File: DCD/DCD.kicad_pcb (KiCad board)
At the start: 4 copper layers, 110 x 110 mm, 172 parts, among them IC1 830S21AMI-01LF, IC2 830S21AMI-01LF, J1 UMPS-04-03.5-G-VT-SM-WT, J2 UMPS-04-03.5-G-VT-SM-WT, J3 UMPS-04-03.5-G-VT-SM-WT, J4 UMPS-04-03.5-G-VT-SM-WT, J5 Conn_02x04_Top_Bottom, U1 TLV76780DBVR, U10 OPA277UA, U11 DAC8811ICDGKT, U12 DAC8811ICDGKT, U13 OPA277UA, U14 OPA277UA, U15 MC100EP31DTG, U16 MC100EP31DTG, U2 ADP7182AUJZ-1.8-R7, U3 LP2985-50DBVR, U4 LP2985-18DBVR, U5 LP2985-33DBVR, U6 ADR4550BRZ, U7 LP2985-33DBVR, U8 CDCLVC1104PWR, U9 AD4630-24BBCZ, Y1 SiT8208AI-21-33E-50.000000

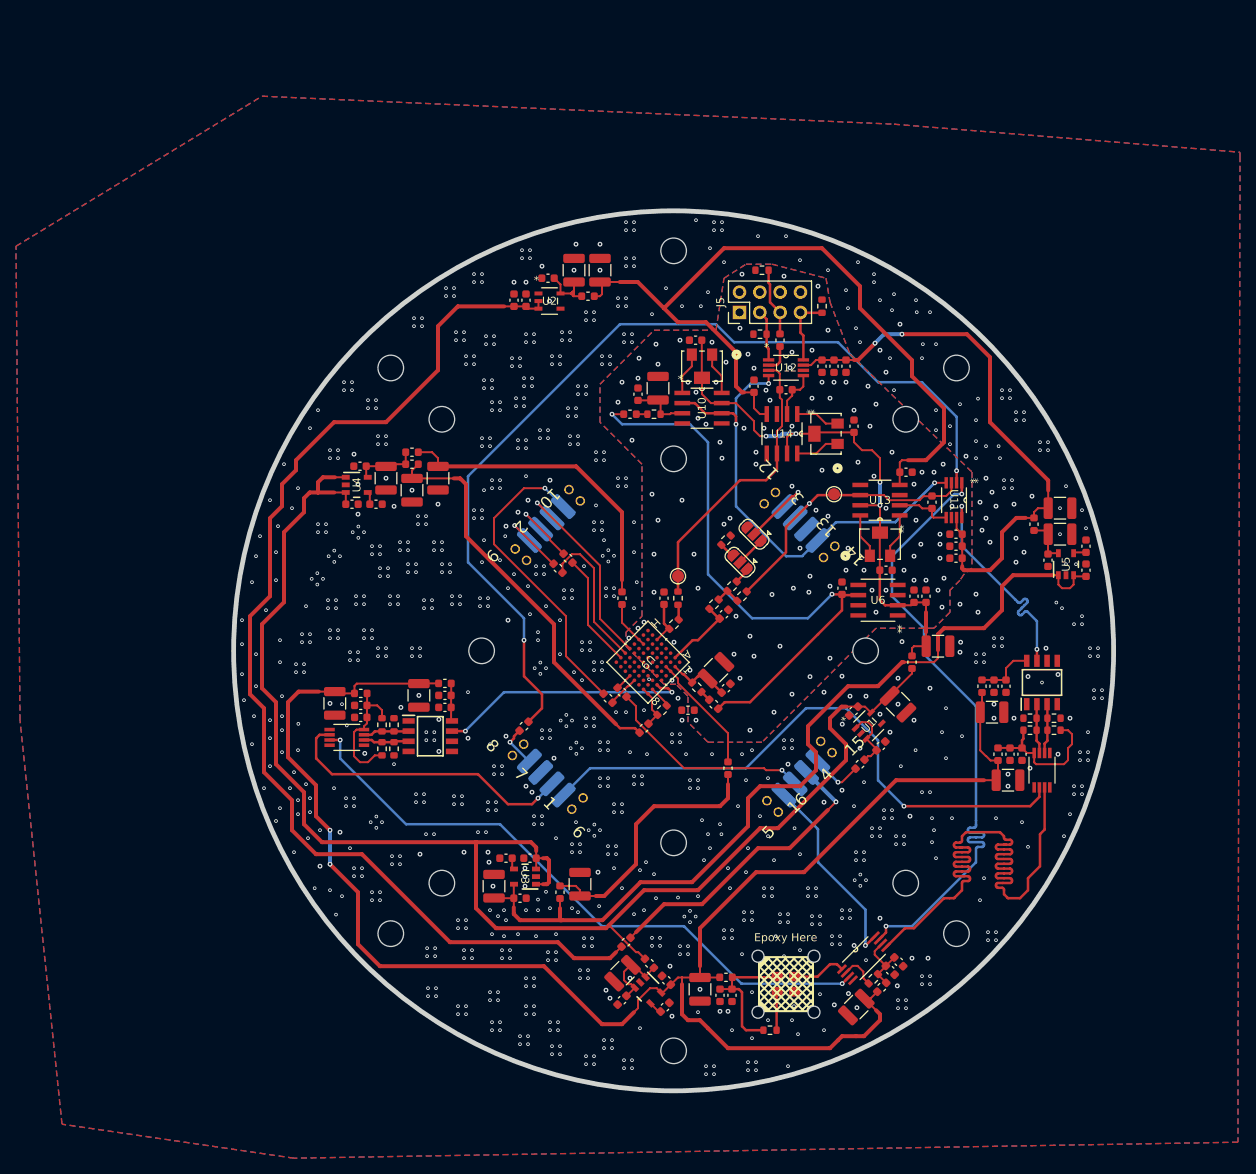
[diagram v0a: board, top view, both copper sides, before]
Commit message: Component placement
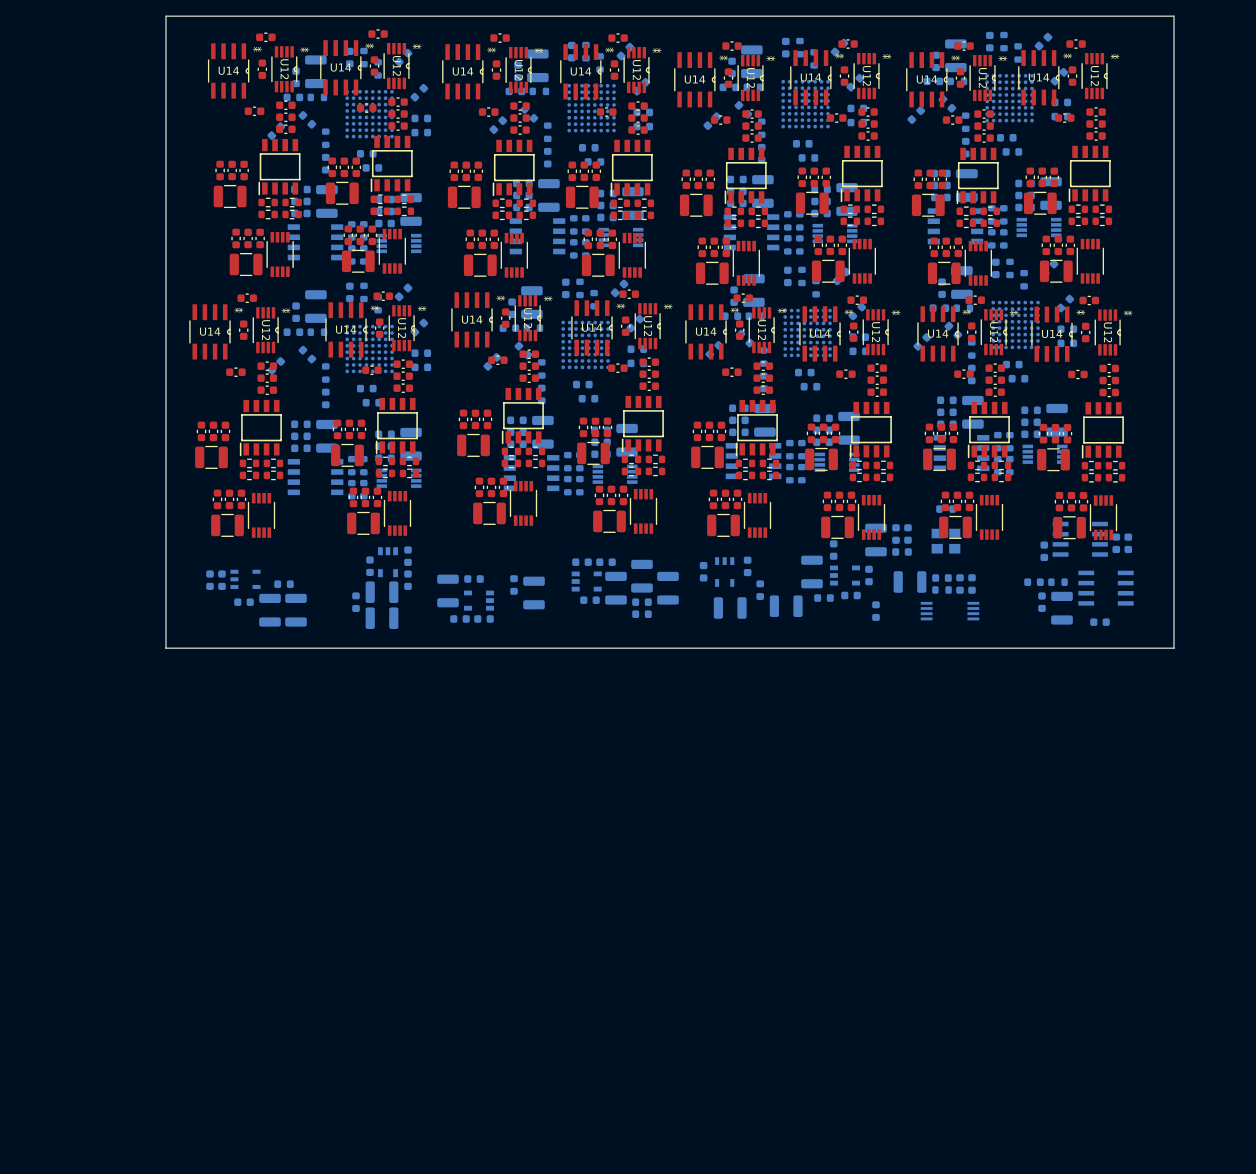
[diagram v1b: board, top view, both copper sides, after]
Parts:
- removed B1: DIN933 M3x14mm, custom_components:Screw_DIN933_M3x14mm
- removed C38: 1µF, Capacitor_SMD:C_0603_1608Metric
- removed C40: 100p, Capacitor_SMD:C_0603_1608Metric
- removed C43: 1nF, Capacitor_SMD:C_0603_1608Metric
- removed C44: 10pF, Capacitor_SMD:C_0603_1608Metric
- removed C47, C48: 100nF, Capacitor_SMD:C_0603_1608Metric
- removed FB11, FB12, FB14: 470Ω, Inductor_SMD:L_0603_1608Metric
- removed H1, H10, H11, H12, H13, H14, H2, H3, H4, H5, H6, H7, H8, H9: M3 Mounting hole, LOBSTER:MountingHole_3.2mm_M3_NoMask
- removed H15: Spacer M3x5mm, custom_components:ThreadedSpacer_6mm_M3x0.5_5mm
- removed J1, J2, J3, J4: UMPS-04-03.5-G-VT-SM-WT, custom_components:UMPS-04-03.5-G-VT-SM-WT
- removed J5: Conn_02x04_Top_Bottom, Connector_PinHeader_2.54mm:PinHeader_2x04_P2.54mm_Vertical
- removed JP1, JP2: SolderJumper_3_Open, Jumper:SolderJumper-3_P1.3mm_Open_RoundedPad1.0x1.5mm
- removed N1, N2, N3, N4, N5, N6, N7: M3 Thumbnut, custom_components:ThumbNut-M3
- removed R17: 47, Resistor_SMD:R_0603_1608Metric
- removed R18, R19, R20: 1k, Resistor_SMD:R_0603_1608Metric
- removed R3, R4, R5: 10k, Resistor_SMD:R_0603_1608Metric
- removed RV1, RV2, RV3: 20kR, custom_components:IC3_3214W-1-203E_BRN
- removed TP1, TP2: TestPoint, TestPoint:TestPoint_Pad_D1.5mm
- removed U11: DAC8811ICDGKT, custom_components:DGK8
- removed U13: OPA277UA, custom_components:D8
- added C23: 10uF, Capacitor_SMD:C_1210_3225Metric, F.Cu at (194.5, 47.6)
- added C23: 10uF, Capacitor_SMD:C_1210_3225Metric, F.Cu at (138.7, 78.9)
- added C23: 10uF, Capacitor_SMD:C_1210_3225Metric, F.Cu at (122.5, 46.9)
- added C23: 10uF, Capacitor_SMD:C_1210_3225Metric, F.Cu at (152.9, 79.4)
- added C23: 10uF, Capacitor_SMD:C_1210_3225Metric, F.Cu at (123.7, 77.9)
- added C23: 10uF, Capacitor_SMD:C_1210_3225Metric, F.Cu at (107.9, 79.2)
- added C23: 10uF, Capacitor_SMD:C_1210_3225Metric, F.Cu at (90.9, 79.4)
- added C23: 10uF, Capacitor_SMD:C_1210_3225Metric, F.Cu at (180.5, 47.9)
- added C23: 10uF, Capacitor_SMD:C_1210_3225Metric, F.Cu at (137.3, 46.9)
- added C23: 10uF, Capacitor_SMD:C_1210_3225Metric, F.Cu at (167.2, 79.7)
- added C23: 10uF, Capacitor_SMD:C_1210_3225Metric, F.Cu at (181.9, 79.7)
- added C23: 10uF, Capacitor_SMD:C_1210_3225Metric, F.Cu at (196.2, 79.7)
- added C23: 10uF, Capacitor_SMD:C_1210_3225Metric, F.Cu at (107.3, 46.4)
- added C23: 10uF, Capacitor_SMD:C_1210_3225Metric, F.Cu at (166.0, 47.6)
- added C23: 10uF, Capacitor_SMD:C_1210_3225Metric, F.Cu at (151.5, 47.9)
- added C30: 10uF, Capacitor_SMD:C_1210_3225Metric, B.Cu at (129.0, 51.5)
- added C30: 10uF, Capacitor_SMD:C_1210_3225Metric, B.Cu at (129.7, 21.9)
- added C30: 10uF, Capacitor_SMD:C_1210_3225Metric, B.Cu at (102.0, 22.7)
- added C30: 10uF, Capacitor_SMD:C_1210_3225Metric, B.Cu at (156.5, 21.4)
- added C30: 10uF, Capacitor_SMD:C_1210_3225Metric, B.Cu at (102.0, 52.0)
- added C30: 10uF, Capacitor_SMD:C_1210_3225Metric, B.Cu at (156.7, 50.0)
- added C30: 10uF, Capacitor_SMD:C_1210_3225Metric, B.Cu at (182.7, 49.0)
- added C32: 100nF, Capacitor_SMD:C_0603_1608Metric, B.Cu at (180.3, 49.8)
- added C32: 100nF, Capacitor_SMD:C_0603_1608Metric, B.Cu at (154.3, 50.8)
- added C32: 100nF, Capacitor_SMD:C_0603_1608Metric, B.Cu at (99.5, 52.8)
- added C32: 100nF, Capacitor_SMD:C_0603_1608Metric, B.Cu at (154.0, 22.2)
- added C32: 100nF, Capacitor_SMD:C_0603_1608Metric, B.Cu at (126.5, 52.2)
- added C32: 100nF, Capacitor_SMD:C_0603_1608Metric, B.Cu at (99.5, 23.4)
- added C32: 100nF, Capacitor_SMD:C_0603_1608Metric, B.Cu at (127.3, 22.7)
- added C36: 1nF, Capacitor_SMD:C_0603_1608Metric, B.Cu at (160.7, 19.7)
- added C36: 1nF, Capacitor_SMD:C_0603_1608Metric, B.Cu at (161.0, 48.3)
- added C36: 1nF, Capacitor_SMD:C_0603_1608Metric, B.Cu at (187.0, 47.3)
- added C36: 1nF, Capacitor_SMD:C_0603_1608Metric, B.Cu at (106.2, 50.3)
- added C36: 1nF, Capacitor_SMD:C_0603_1608Metric, B.Cu at (133.2, 49.8)
- added C36: 1nF, Capacitor_SMD:C_0603_1608Metric, B.Cu at (106.2, 20.9)
- added C36: 1nF, Capacitor_SMD:C_0603_1608Metric, B.Cu at (134.0, 20.2)
- added C37: 1nF, Capacitor_SMD:C_0603_1608Metric, B.Cu at (140.7, 20.2)
- added C37: 1nF, Capacitor_SMD:C_0603_1608Metric, B.Cu at (167.4, 19.7)
- added C37: 1nF, Capacitor_SMD:C_0603_1608Metric, B.Cu at (112.9, 50.3)
- added C37: 1nF, Capacitor_SMD:C_0603_1608Metric, B.Cu at (167.7, 48.3)
- added C37: 1nF, Capacitor_SMD:C_0603_1608Metric, B.Cu at (139.9, 49.8)
- added C37: 1nF, Capacitor_SMD:C_0603_1608Metric, B.Cu at (112.9, 20.9)
- added C37: 1nF, Capacitor_SMD:C_0603_1608Metric, B.Cu at (193.7, 47.3)
- added C39: 1µF, Capacitor_SMD:C_0603_1608Metric, F.Cu at (201.2, 62.8)
- added C39: 1µF, Capacitor_SMD:C_0603_1608Metric, F.Cu at (112.9, 62.2)
- added C39: 1µF, Capacitor_SMD:C_0603_1608Metric, F.Cu at (156.5, 31.0)
- added C39: 1µF, Capacitor_SMD:C_0603_1608Metric, F.Cu at (95.9, 62.5)
- added C39: 1µF, Capacitor_SMD:C_0603_1608Metric, F.Cu at (143.7, 62.0)
- added C39: 1µF, Capacitor_SMD:C_0603_1608Metric, F.Cu at (127.5, 30.0)
- added C39: 1µF, Capacitor_SMD:C_0603_1608Metric, F.Cu at (157.9, 62.5)
- added C39: 1µF, Capacitor_SMD:C_0603_1608Metric, F.Cu at (172.2, 62.7)
- added C39: 1µF, Capacitor_SMD:C_0603_1608Metric, F.Cu at (128.7, 61.0)
- added C39: 1µF, Capacitor_SMD:C_0603_1608Metric, F.Cu at (171.0, 30.7)
- added C39: 1µF, Capacitor_SMD:C_0603_1608Metric, F.Cu at (112.3, 29.5)
- added C39: 1µF, Capacitor_SMD:C_0603_1608Metric, F.Cu at (199.5, 30.7)
- added C39: 1µF, Capacitor_SMD:C_0603_1608Metric, F.Cu at (142.3, 30.0)
- added C39: 1µF, Capacitor_SMD:C_0603_1608Metric, F.Cu at (186.9, 62.7)
- added C39: 1µF, Capacitor_SMD:C_0603_1608Metric, F.Cu at (185.5, 31.0)
- added C41: 100p, Capacitor_SMD:C_0603_1608Metric, F.Cu at (112.3, 26.5)
- added C41: 100p, Capacitor_SMD:C_0603_1608Metric, F.Cu at (143.7, 59.0)
- added C41: 100p, Capacitor_SMD:C_0603_1608Metric, F.Cu at (142.3, 27.0)
- added C41: 100p, Capacitor_SMD:C_0603_1608Metric, F.Cu at (156.5, 28.0)
- added C41: 100p, Capacitor_SMD:C_0603_1608Metric, F.Cu at (157.9, 59.5)
- added C41: 100p, Capacitor_SMD:C_0603_1608Metric, F.Cu at (128.7, 58.0)
- added C41: 100p, Capacitor_SMD:C_0603_1608Metric, F.Cu at (186.9, 59.7)
- added C41: 100p, Capacitor_SMD:C_0603_1608Metric, F.Cu at (171.0, 27.7)
- added C41: 100p, Capacitor_SMD:C_0603_1608Metric, F.Cu at (112.9, 59.2)
- added C41: 100p, Capacitor_SMD:C_0603_1608Metric, F.Cu at (95.9, 59.5)
- added C41: 100p, Capacitor_SMD:C_0603_1608Metric, F.Cu at (201.2, 59.8)
- added C41: 100p, Capacitor_SMD:C_0603_1608Metric, F.Cu at (172.2, 59.7)
- added C41: 100p, Capacitor_SMD:C_0603_1608Metric, F.Cu at (127.5, 27.0)
- added C41: 100p, Capacitor_SMD:C_0603_1608Metric, F.Cu at (199.5, 27.7)
- added C41: 100p, Capacitor_SMD:C_0603_1608Metric, F.Cu at (185.5, 28.0)
- added C42: 1nF, Capacitor_SMD:C_0603_1608Metric, F.Cu at (199.5, 29.2)
- added C42: 1nF, Capacitor_SMD:C_0603_1608Metric, F.Cu at (128.7, 59.5)
- added C42: 1nF, Capacitor_SMD:C_0603_1608Metric, F.Cu at (185.5, 29.5)
- added C42: 1nF, Capacitor_SMD:C_0603_1608Metric, F.Cu at (95.9, 61.0)
- added C42: 1nF, Capacitor_SMD:C_0603_1608Metric, F.Cu at (201.2, 61.3)
- added C42: 1nF, Capacitor_SMD:C_0603_1608Metric, F.Cu at (143.7, 60.5)
- added C42: 1nF, Capacitor_SMD:C_0603_1608Metric, F.Cu at (112.9, 60.7)
- added C42: 1nF, Capacitor_SMD:C_0603_1608Metric, F.Cu at (172.2, 61.2)
- added C42: 1nF, Capacitor_SMD:C_0603_1608Metric, F.Cu at (171.0, 29.2)
- added C42: 1nF, Capacitor_SMD:C_0603_1608Metric, F.Cu at (157.9, 61.0)
- added C42: 1nF, Capacitor_SMD:C_0603_1608Metric, F.Cu at (156.5, 29.5)
- added C42: 1nF, Capacitor_SMD:C_0603_1608Metric, F.Cu at (142.3, 28.5)
- added C42: 1nF, Capacitor_SMD:C_0603_1608Metric, F.Cu at (127.5, 28.5)
- added C42: 1nF, Capacitor_SMD:C_0603_1608Metric, F.Cu at (112.3, 28.0)
- added C42: 1nF, Capacitor_SMD:C_0603_1608Metric, F.Cu at (186.9, 61.2)
- added C45: 10pF, Capacitor_SMD:C_0603_1608Metric, F.Cu at (196.6, 23.2)
- added C45: 10pF, Capacitor_SMD:C_0603_1608Metric, F.Cu at (109.3, 22.0)
- added C45: 10pF, Capacitor_SMD:C_0603_1608Metric, F.Cu at (124.6, 22.5)
- added C45: 10pF, Capacitor_SMD:C_0603_1608Metric, F.Cu at (125.7, 53.5)
- added C45: 10pF, Capacitor_SMD:C_0603_1608Metric, F.Cu at (93.0, 55.0)
- added C45: 10pF, Capacitor_SMD:C_0603_1608Metric, F.Cu at (155.0, 55.0)
- added C45: 10pF, Capacitor_SMD:C_0603_1608Metric, F.Cu at (139.3, 22.5)
- added C45: 10pF, Capacitor_SMD:C_0603_1608Metric, F.Cu at (184.0, 55.2)
- added C45: 10pF, Capacitor_SMD:C_0603_1608Metric, F.Cu at (169.2, 55.2)
- added C45: 10pF, Capacitor_SMD:C_0603_1608Metric, F.Cu at (140.7, 54.5)
- added C45: 10pF, Capacitor_SMD:C_0603_1608Metric, F.Cu at (182.6, 23.5)
- added C45: 10pF, Capacitor_SMD:C_0603_1608Metric, F.Cu at (110.0, 54.7)
- added C45: 10pF, Capacitor_SMD:C_0603_1608Metric, F.Cu at (153.6, 23.5)
- added C45: 10pF, Capacitor_SMD:C_0603_1608Metric, F.Cu at (198.2, 55.3)
- added C45: 10pF, Capacitor_SMD:C_0603_1608Metric, F.Cu at (168.1, 23.2)
- added C49: 100nF, Capacitor_SMD:C_0603_1608Metric, F.Cu at (141.2, 50.5)
- added C49: 100nF, Capacitor_SMD:C_0603_1608Metric, F.Cu at (109.8, 18.0)
- added C49: 100nF, Capacitor_SMD:C_0603_1608Metric, F.Cu at (169.7, 51.2)
- added C49: 100nF, Capacitor_SMD:C_0603_1608Metric, F.Cu at (168.5, 19.2)
- added C49: 100nF, Capacitor_SMD:C_0603_1608Metric, F.Cu at (198.7, 51.3)
- added C49: 100nF, Capacitor_SMD:C_0603_1608Metric, F.Cu at (197.0, 19.2)
- added C49: 100nF, Capacitor_SMD:C_0603_1608Metric, F.Cu at (125.0, 18.5)
- added C49: 100nF, Capacitor_SMD:C_0603_1608Metric, F.Cu at (154.0, 19.5)
- added C49: 100nF, Capacitor_SMD:C_0603_1608Metric, F.Cu at (184.4, 51.2)
- added C49: 100nF, Capacitor_SMD:C_0603_1608Metric, F.Cu at (155.4, 51.0)
- added C49: 100nF, Capacitor_SMD:C_0603_1608Metric, F.Cu at (139.8, 18.5)
- added C49: 100nF, Capacitor_SMD:C_0603_1608Metric, F.Cu at (93.4, 51.0)
- added C49: 100nF, Capacitor_SMD:C_0603_1608Metric, F.Cu at (183.0, 19.5)
- added C49: 100nF, Capacitor_SMD:C_0603_1608Metric, F.Cu at (110.4, 50.7)
- added C50: 100nF, Capacitor_SMD:C_0603_1608Metric, F.Cu at (181.6, 28.7)
- added C50: 100nF, Capacitor_SMD:C_0603_1608Metric, F.Cu at (109.0, 60.0)
- added C50: 100nF, Capacitor_SMD:C_0603_1608Metric, F.Cu at (168.2, 60.5)
- added C50: 100nF, Capacitor_SMD:C_0603_1608Metric, F.Cu at (197.2, 60.5)
- added C50: 100nF, Capacitor_SMD:C_0603_1608Metric, F.Cu at (139.7, 59.7)
- added C50: 100nF, Capacitor_SMD:C_0603_1608Metric, F.Cu at (183.0, 60.5)
- added C50: 100nF, Capacitor_SMD:C_0603_1608Metric, F.Cu at (92.0, 60.2)
- added C50: 100nF, Capacitor_SMD:C_0603_1608Metric, F.Cu at (154.0, 60.2)
- added C50: 100nF, Capacitor_SMD:C_0603_1608Metric, F.Cu at (108.3, 27.2)
- added C50: 100nF, Capacitor_SMD:C_0603_1608Metric, F.Cu at (138.3, 27.7)
- added C50: 100nF, Capacitor_SMD:C_0603_1608Metric, F.Cu at (123.6, 27.7)
- added C50: 100nF, Capacitor_SMD:C_0603_1608Metric, F.Cu at (167.1, 28.5)
- added C50: 100nF, Capacitor_SMD:C_0603_1608Metric, F.Cu at (195.6, 28.5)
- added C50: 100nF, Capacitor_SMD:C_0603_1608Metric, F.Cu at (124.7, 58.7)
- added C50: 100nF, Capacitor_SMD:C_0603_1608Metric, F.Cu at (152.6, 28.7)
- added C59: 1µF, Capacitor_SMD:C_0603_1608Metric, F.Cu at (138.9, 75.7)
- added C59: 1µF, Capacitor_SMD:C_0603_1608Metric, F.Cu at (182.2, 76.4)
- added C59: 1µF, Capacitor_SMD:C_0603_1608Metric, F.Cu at (167.4, 76.4)
- added C59: 1µF, Capacitor_SMD:C_0603_1608Metric, F.Cu at (151.8, 44.6)
- added C59: 1µF, Capacitor_SMD:C_0603_1608Metric, F.Cu at (180.8, 44.6)
- added C59: 1µF, Capacitor_SMD:C_0603_1608Metric, F.Cu at (108.2, 75.9)
- added C59: 1µF, Capacitor_SMD:C_0603_1608Metric, F.Cu at (137.5, 43.6)
- added C59: 1µF, Capacitor_SMD:C_0603_1608Metric, F.Cu at (153.2, 76.2)
- added C59: 1µF, Capacitor_SMD:C_0603_1608Metric, F.Cu at (123.9, 74.7)
- added C59: 1µF, Capacitor_SMD:C_0603_1608Metric, F.Cu at (91.2, 76.2)
- added C59: 1µF, Capacitor_SMD:C_0603_1608Metric, F.Cu at (194.8, 44.4)
- added C59: 1µF, Capacitor_SMD:C_0603_1608Metric, F.Cu at (107.5, 43.1)
- added C59: 1µF, Capacitor_SMD:C_0603_1608Metric, F.Cu at (122.8, 43.6)
- added C59: 1µF, Capacitor_SMD:C_0603_1608Metric, F.Cu at (196.4, 76.4)
- added C59: 1µF, Capacitor_SMD:C_0603_1608Metric, F.Cu at (166.3, 44.4)
- added C60: 100nF, Capacitor_SMD:C_0603_1608Metric, F.Cu at (153.3, 44.6)
- added C60: 100nF, Capacitor_SMD:C_0603_1608Metric, F.Cu at (92.7, 76.2)
- added C60: 100nF, Capacitor_SMD:C_0603_1608Metric, F.Cu at (167.8, 44.4)
- added C60: 100nF, Capacitor_SMD:C_0603_1608Metric, F.Cu at (109.0, 43.1)
- added C60: 100nF, Capacitor_SMD:C_0603_1608Metric, F.Cu at (139.0, 43.6)
- added C60: 100nF, Capacitor_SMD:C_0603_1608Metric, F.Cu at (109.7, 75.9)
- added C60: 100nF, Capacitor_SMD:C_0603_1608Metric, F.Cu at (140.4, 75.7)
- added C60: 100nF, Capacitor_SMD:C_0603_1608Metric, F.Cu at (124.3, 43.6)
- added C60: 100nF, Capacitor_SMD:C_0603_1608Metric, F.Cu at (183.7, 76.4)
- added C60: 100nF, Capacitor_SMD:C_0603_1608Metric, F.Cu at (154.7, 76.2)
- added C60: 100nF, Capacitor_SMD:C_0603_1608Metric, F.Cu at (197.9, 76.4)
- added C60: 100nF, Capacitor_SMD:C_0603_1608Metric, F.Cu at (168.9, 76.4)
- added C60: 100nF, Capacitor_SMD:C_0603_1608Metric, F.Cu at (196.3, 44.4)
- added C60: 100nF, Capacitor_SMD:C_0603_1608Metric, F.Cu at (125.4, 74.7)
- added C60: 100nF, Capacitor_SMD:C_0603_1608Metric, F.Cu at (182.3, 44.6)
- added C61: 10uF, Capacitor_SMD:C_1210_3225Metric, F.Cu at (136.7, 70.4)
- added C61: 10uF, Capacitor_SMD:C_1210_3225Metric, F.Cu at (120.5, 38.4)
- added C61: 10uF, Capacitor_SMD:C_1210_3225Metric, F.Cu at (149.5, 39.4)
- added C61: 10uF, Capacitor_SMD:C_1210_3225Metric, F.Cu at (88.9, 70.9)
- added C61: 10uF, Capacitor_SMD:C_1210_3225Metric, F.Cu at (121.7, 69.4)
- added C61: 10uF, Capacitor_SMD:C_1210_3225Metric, F.Cu at (178.5, 39.4)
- added C61: 10uF, Capacitor_SMD:C_1210_3225Metric, F.Cu at (135.3, 38.4)
- added C61: 10uF, Capacitor_SMD:C_1210_3225Metric, F.Cu at (165.2, 71.2)
- added C61: 10uF, Capacitor_SMD:C_1210_3225Metric, F.Cu at (105.3, 37.9)
- added C61: 10uF, Capacitor_SMD:C_1210_3225Metric, F.Cu at (179.9, 71.2)
- added C61: 10uF, Capacitor_SMD:C_1210_3225Metric, F.Cu at (150.9, 70.9)
- added C61: 10uF, Capacitor_SMD:C_1210_3225Metric, F.Cu at (105.9, 70.7)
- added C61: 10uF, Capacitor_SMD:C_1210_3225Metric, F.Cu at (164.0, 39.1)
- added C61: 10uF, Capacitor_SMD:C_1210_3225Metric, F.Cu at (194.2, 71.2)
- added C61: 10uF, Capacitor_SMD:C_1210_3225Metric, F.Cu at (192.5, 39.1)
- added C62: 1µF, Capacitor_SMD:C_0603_1608Metric, F.Cu at (151.2, 67.7)
- added C62: 1µF, Capacitor_SMD:C_0603_1608Metric, F.Cu at (105.5, 34.6)
- added C62: 1µF, Capacitor_SMD:C_0603_1608Metric, F.Cu at (120.8, 35.1)
- added C62: 1µF, Capacitor_SMD:C_0603_1608Metric, F.Cu at (89.2, 67.7)
- added C62: 1µF, Capacitor_SMD:C_0603_1608Metric, F.Cu at (165.4, 67.9)
- added C62: 1µF, Capacitor_SMD:C_0603_1608Metric, F.Cu at (192.8, 35.9)
- added C62: 1µF, Capacitor_SMD:C_0603_1608Metric, F.Cu at (194.4, 67.9)
- added C62: 1µF, Capacitor_SMD:C_0603_1608Metric, F.Cu at (178.8, 36.1)
- added C62: 1µF, Capacitor_SMD:C_0603_1608Metric, F.Cu at (106.2, 67.4)
- added C62: 1µF, Capacitor_SMD:C_0603_1608Metric, F.Cu at (121.9, 66.2)
- added C62: 1µF, Capacitor_SMD:C_0603_1608Metric, F.Cu at (135.5, 35.1)
- added C62: 1µF, Capacitor_SMD:C_0603_1608Metric, F.Cu at (149.8, 36.1)
- added C62: 1µF, Capacitor_SMD:C_0603_1608Metric, F.Cu at (164.3, 35.9)
- added C62: 1µF, Capacitor_SMD:C_0603_1608Metric, F.Cu at (180.2, 67.9)
- added C62: 1µF, Capacitor_SMD:C_0603_1608Metric, F.Cu at (136.9, 67.2)
- added C63: 100nF, Capacitor_SMD:C_0603_1608Metric, F.Cu at (180.3, 36.1)
- added C63: 100nF, Capacitor_SMD:C_0603_1608Metric, F.Cu at (166.9, 67.9)
- added C63: 100nF, Capacitor_SMD:C_0603_1608Metric, F.Cu at (107.0, 34.6)
- added C63: 100nF, Capacitor_SMD:C_0603_1608Metric, F.Cu at (138.4, 67.2)
- added C63: 100nF, Capacitor_SMD:C_0603_1608Metric, F.Cu at (165.8, 35.9)
- added C63: 100nF, Capacitor_SMD:C_0603_1608Metric, F.Cu at (194.3, 35.9)
- added C63: 100nF, Capacitor_SMD:C_0603_1608Metric, F.Cu at (123.4, 66.2)
- added C63: 100nF, Capacitor_SMD:C_0603_1608Metric, F.Cu at (195.9, 67.9)
- added C63: 100nF, Capacitor_SMD:C_0603_1608Metric, F.Cu at (181.7, 67.9)
- added C63: 100nF, Capacitor_SMD:C_0603_1608Metric, F.Cu at (90.7, 67.7)
- added C63: 100nF, Capacitor_SMD:C_0603_1608Metric, F.Cu at (137.0, 35.1)
- added C63: 100nF, Capacitor_SMD:C_0603_1608Metric, F.Cu at (151.3, 36.1)
- added C63: 100nF, Capacitor_SMD:C_0603_1608Metric, F.Cu at (107.7, 67.4)
- added C63: 100nF, Capacitor_SMD:C_0603_1608Metric, F.Cu at (152.7, 67.7)
- added C63: 100nF, Capacitor_SMD:C_0603_1608Metric, F.Cu at (122.3, 35.1)
- added C64: 10uF, Capacitor_SMD:C_1210_3225Metric, B.Cu at (168.4, 38.7)
- added C64: 10uF, Capacitor_SMD:C_1210_3225Metric, B.Cu at (141.6, 39.2)
- added C64: 10uF, Capacitor_SMD:C_1210_3225Metric, B.Cu at (168.6, 67.3)
- added C64: 10uF, Capacitor_SMD:C_1210_3225Metric, B.Cu at (113.9, 69.3)
- added C64: 10uF, Capacitor_SMD:C_1210_3225Metric, B.Cu at (113.9, 39.9)
- added C64: 10uF, Capacitor_SMD:C_1210_3225Metric, B.Cu at (140.9, 68.8)
- added C64: 10uF, Capacitor_SMD:C_1210_3225Metric, B.Cu at (194.6, 66.3)
- added C65: 1µF, Capacitor_SMD:C_0603_1608Metric, B.Cu at (110.6, 40.2)
- added C65: 1µF, Capacitor_SMD:C_0603_1608Metric, B.Cu at (138.4, 39.4)
- added C65: 1µF, Capacitor_SMD:C_0603_1608Metric, B.Cu at (191.4, 66.5)
- added C65: 1µF, Capacitor_SMD:C_0603_1608Metric, B.Cu at (137.6, 69.0)
- added C65: 1µF, Capacitor_SMD:C_0603_1608Metric, B.Cu at (165.4, 67.5)
- added C65: 1µF, Capacitor_SMD:C_0603_1608Metric, B.Cu at (110.6, 69.5)
- added C65: 1µF, Capacitor_SMD:C_0603_1608Metric, B.Cu at (165.1, 38.9)
- added C66: 100nF, Capacitor_SMD:C_0603_1608Metric, B.Cu at (138.4, 40.9)
- added C66: 100nF, Capacitor_SMD:C_0603_1608Metric, B.Cu at (165.4, 69.0)
- added C66: 100nF, Capacitor_SMD:C_0603_1608Metric, B.Cu at (110.6, 71.0)
- added C66: 100nF, Capacitor_SMD:C_0603_1608Metric, B.Cu at (137.6, 70.5)
- added C66: 100nF, Capacitor_SMD:C_0603_1608Metric, B.Cu at (191.4, 68.0)
- added C66: 100nF, Capacitor_SMD:C_0603_1608Metric, B.Cu at (165.1, 40.4)
- added C66: 100nF, Capacitor_SMD:C_0603_1608Metric, B.Cu at (110.6, 41.7)
- added C67: 100nF, Capacitor_SMD:C_0603_1608Metric, B.Cu at (180.9, 66.8)
- added C67: 100nF, Capacitor_SMD:C_0603_1608Metric, B.Cu at (100.1, 69.8)
- added C67: 100nF, Capacitor_SMD:C_0603_1608Metric, B.Cu at (154.9, 67.8)
- added C67: 100nF, Capacitor_SMD:C_0603_1608Metric, B.Cu at (154.6, 39.2)
- added C67: 100nF, Capacitor_SMD:C_0603_1608Metric, B.Cu at (127.9, 39.7)
- added C67: 100nF, Capacitor_SMD:C_0603_1608Metric, B.Cu at (127.1, 69.3)
- added C67: 100nF, Capacitor_SMD:C_0603_1608Metric, B.Cu at (100.1, 40.4)
- added C68: 1µF, Capacitor_SMD:C_0603_1608Metric, B.Cu at (180.9, 65.3)
- added C68: 1µF, Capacitor_SMD:C_0603_1608Metric, B.Cu at (100.1, 38.9)
- added C68: 1µF, Capacitor_SMD:C_0603_1608Metric, B.Cu at (127.1, 67.8)
- added C68: 1µF, Capacitor_SMD:C_0603_1608Metric, B.Cu at (154.9, 66.3)
- added C68: 1µF, Capacitor_SMD:C_0603_1608Metric, B.Cu at (100.1, 68.3)
- added C68: 1µF, Capacitor_SMD:C_0603_1608Metric, B.Cu at (154.6, 37.7)
- added C68: 1µF, Capacitor_SMD:C_0603_1608Metric, B.Cu at (127.9, 38.2)
- added C69: 10uF, Capacitor_SMD:C_1210_3225Metric, B.Cu at (157.9, 37.7)
- added C69: 10uF, Capacitor_SMD:C_1210_3225Metric, B.Cu at (158.1, 66.3)
- added C69: 10uF, Capacitor_SMD:C_1210_3225Metric, B.Cu at (103.4, 38.9)
- added C69: 10uF, Capacitor_SMD:C_1210_3225Metric, B.Cu at (131.1, 38.2)
- added C69: 10uF, Capacitor_SMD:C_1210_3225Metric, B.Cu at (103.4, 68.3)
- added C69: 10uF, Capacitor_SMD:C_1210_3225Metric, B.Cu at (184.1, 65.3)
- added C69: 10uF, Capacitor_SMD:C_1210_3225Metric, B.Cu at (130.4, 67.8)
- added FB10: 470Ω, Inductor_SMD:L_0603_1608Metric, B.Cu at (136.1, 32.2)
- added FB10: 470Ω, Inductor_SMD:L_0603_1608Metric, B.Cu at (108.3, 32.9)
- added FB10: 470Ω, Inductor_SMD:L_0603_1608Metric, B.Cu at (163.1, 60.3)
- added FB10: 470Ω, Inductor_SMD:L_0603_1608Metric, B.Cu at (189.1, 59.3)
- added FB10: 470Ω, Inductor_SMD:L_0603_1608Metric, B.Cu at (162.8, 31.7)
- added FB10: 470Ω, Inductor_SMD:L_0603_1608Metric, B.Cu at (108.3, 62.3)
- added FB10: 470Ω, Inductor_SMD:L_0603_1608Metric, B.Cu at (135.3, 61.8)
- added FB13: 470Ω, Inductor_SMD:L_0603_1608Metric, B.Cu at (115.2, 57.9)
- added FB13: 470Ω, Inductor_SMD:L_0603_1608Metric, B.Cu at (169.9, 55.9)
- added FB13: 470Ω, Inductor_SMD:L_0603_1608Metric, B.Cu at (142.9, 27.8)
- added FB13: 470Ω, Inductor_SMD:L_0603_1608Metric, B.Cu at (195.9, 54.9)
- added FB13: 470Ω, Inductor_SMD:L_0603_1608Metric, B.Cu at (142.2, 57.4)
- added FB13: 470Ω, Inductor_SMD:L_0603_1608Metric, B.Cu at (115.2, 28.5)
- added FB13: 470Ω, Inductor_SMD:L_0603_1608Metric, B.Cu at (169.7, 27.3)
- added FB16: 470Ω, Inductor_SMD:L_0603_1608Metric, B.Cu at (115.2, 59.6)
- added FB16: 470Ω, Inductor_SMD:L_0603_1608Metric, B.Cu at (195.9, 56.6)
- added FB16: 470Ω, Inductor_SMD:L_0603_1608Metric, B.Cu at (169.7, 29.0)
- added FB16: 470Ω, Inductor_SMD:L_0603_1608Metric, B.Cu at (169.9, 57.6)
- added FB16: 470Ω, Inductor_SMD:L_0603_1608Metric, B.Cu at (142.9, 29.5)
- added FB16: 470Ω, Inductor_SMD:L_0603_1608Metric, B.Cu at (115.2, 30.3)
- added FB16: 470Ω, Inductor_SMD:L_0603_1608Metric, B.Cu at (142.2, 59.1)
- added FB20: 470Ω, Inductor_SMD:L_0603_1608Metric, B.Cu at (100.9, 28.7)
- added FB20: 470Ω, Inductor_SMD:L_0603_1608Metric, B.Cu at (181.7, 55.1)
- added FB20: 470Ω, Inductor_SMD:L_0603_1608Metric, B.Cu at (100.9, 58.1)
- added FB20: 470Ω, Inductor_SMD:L_0603_1608Metric, B.Cu at (127.9, 57.6)
- added FB20: 470Ω, Inductor_SMD:L_0603_1608Metric, B.Cu at (155.4, 27.5)
- added FB20: 470Ω, Inductor_SMD:L_0603_1608Metric, B.Cu at (155.7, 56.1)
- added FB20: 470Ω, Inductor_SMD:L_0603_1608Metric, B.Cu at (128.7, 28.0)
- added FB22: 470Ω, Inductor_SMD:L_0603_1608Metric, B.Cu at (103.2, 34.2)
- added FB22: 470Ω, Inductor_SMD:L_0603_1608Metric, B.Cu at (130.2, 63.0)
- added FB22: 470Ω, Inductor_SMD:L_0603_1608Metric, B.Cu at (158.0, 61.5)
- added FB22: 470Ω, Inductor_SMD:L_0603_1608Metric, B.Cu at (184.0, 60.5)
- added FB22: 470Ω, Inductor_SMD:L_0603_1608Metric, B.Cu at (157.7, 32.9)
- added FB22: 470Ω, Inductor_SMD:L_0603_1608Metric, B.Cu at (103.2, 63.5)
- added FB22: 470Ω, Inductor_SMD:L_0603_1608Metric, B.Cu at (131.0, 33.4)
- added FB23: 470Ω, Inductor_SMD:L_0603_1608Metric, B.Cu at (169.7, 52.7)
- added FB23: 470Ω, Inductor_SMD:L_0603_1608Metric, B.Cu at (141.9, 54.2)
- added FB23: 470Ω, Inductor_SMD:L_0603_1608Metric, B.Cu at (114.9, 54.7)
- added FB23: 470Ω, Inductor_SMD:L_0603_1608Metric, B.Cu at (142.7, 24.6)
- added FB23: 470Ω, Inductor_SMD:L_0603_1608Metric, B.Cu at (169.4, 24.1)
- added FB23: 470Ω, Inductor_SMD:L_0603_1608Metric, B.Cu at (114.9, 25.3)
- added FB23: 470Ω, Inductor_SMD:L_0603_1608Metric, B.Cu at (195.7, 51.7)
- added FB24: 470Ω, Inductor_SMD:L_0603_1608Metric, B.Cu at (124.8, 29.4)
- added FB24: 470Ω, Inductor_SMD:L_0603_1608Metric, B.Cu at (177.8, 56.5)
- added FB24: 470Ω, Inductor_SMD:L_0603_1608Metric, B.Cu at (151.5, 28.9)
- added FB24: 470Ω, Inductor_SMD:L_0603_1608Metric, B.Cu at (97.0, 59.5)
- added FB24: 470Ω, Inductor_SMD:L_0603_1608Metric, B.Cu at (97.0, 30.1)
- added FB24: 470Ω, Inductor_SMD:L_0603_1608Metric, B.Cu at (151.8, 57.5)
- added FB24: 470Ω, Inductor_SMD:L_0603_1608Metric, B.Cu at (124.0, 59.0)
- added FB26: 470Ω, Inductor_SMD:L_0603_1608Metric, F.Cu at (151.7, 76.2)
- added FB26: 470Ω, Inductor_SMD:L_0603_1608Metric, F.Cu at (150.3, 44.6)
- added FB26: 470Ω, Inductor_SMD:L_0603_1608Metric, F.Cu at (106.7, 75.9)
- added FB26: 470Ω, Inductor_SMD:L_0603_1608Metric, F.Cu at (136.0, 43.6)
- added FB26: 470Ω, Inductor_SMD:L_0603_1608Metric, F.Cu at (180.7, 76.4)
- added FB26: 470Ω, Inductor_SMD:L_0603_1608Metric, F.Cu at (179.3, 44.6)
- added FB26: 470Ω, Inductor_SMD:L_0603_1608Metric, F.Cu at (122.4, 74.7)
- added FB26: 470Ω, Inductor_SMD:L_0603_1608Metric, F.Cu at (121.3, 43.6)
- added FB26: 470Ω, Inductor_SMD:L_0603_1608Metric, F.Cu at (165.9, 76.4)
- added FB26: 470Ω, Inductor_SMD:L_0603_1608Metric, F.Cu at (137.4, 75.7)
- added FB26: 470Ω, Inductor_SMD:L_0603_1608Metric, F.Cu at (193.3, 44.4)
- added FB26: 470Ω, Inductor_SMD:L_0603_1608Metric, F.Cu at (106.0, 43.1)
- added FB26: 470Ω, Inductor_SMD:L_0603_1608Metric, F.Cu at (89.7, 76.2)
- added FB26: 470Ω, Inductor_SMD:L_0603_1608Metric, F.Cu at (194.9, 76.4)
- added FB26: 470Ω, Inductor_SMD:L_0603_1608Metric, F.Cu at (164.8, 44.4)
- added FB27: 470Ω, Inductor_SMD:L_0603_1608Metric, F.Cu at (87.7, 67.7)
- added FB27: 470Ω, Inductor_SMD:L_0603_1608Metric, F.Cu at (148.3, 36.1)
- added FB27: 470Ω, Inductor_SMD:L_0603_1608Metric, F.Cu at (163.9, 67.9)
- added FB27: 470Ω, Inductor_SMD:L_0603_1608Metric, F.Cu at (104.7, 67.4)
- added FB27: 470Ω, Inductor_SMD:L_0603_1608Metric, F.Cu at (192.9, 67.9)
- added FB27: 470Ω, Inductor_SMD:L_0603_1608Metric, F.Cu at (119.3, 35.1)
- added FB27: 470Ω, Inductor_SMD:L_0603_1608Metric, F.Cu at (134.0, 35.1)
- added FB27: 470Ω, Inductor_SMD:L_0603_1608Metric, F.Cu at (162.8, 35.9)
- added FB27: 470Ω, Inductor_SMD:L_0603_1608Metric, F.Cu at (149.7, 67.7)
- added FB27: 470Ω, Inductor_SMD:L_0603_1608Metric, F.Cu at (120.4, 66.2)
- added FB27: 470Ω, Inductor_SMD:L_0603_1608Metric, F.Cu at (178.7, 67.9)
- added FB27: 470Ω, Inductor_SMD:L_0603_1608Metric, F.Cu at (104.0, 34.6)
- added FB27: 470Ω, Inductor_SMD:L_0603_1608Metric, F.Cu at (177.3, 36.1)
- added FB27: 470Ω, Inductor_SMD:L_0603_1608Metric, F.Cu at (191.3, 35.9)
- added FB27: 470Ω, Inductor_SMD:L_0603_1608Metric, F.Cu at (135.4, 67.2)
- added FB28: 470Ω, Inductor_SMD:L_0603_1608Metric, B.Cu at (110.6, 68.0)
- added FB28: 470Ω, Inductor_SMD:L_0603_1608Metric, B.Cu at (165.1, 37.4)
- added FB28: 470Ω, Inductor_SMD:L_0603_1608Metric, B.Cu at (165.4, 66.0)
- added FB28: 470Ω, Inductor_SMD:L_0603_1608Metric, B.Cu at (137.6, 67.5)
- added FB28: 470Ω, Inductor_SMD:L_0603_1608Metric, B.Cu at (138.4, 37.9)
- added FB28: 470Ω, Inductor_SMD:L_0603_1608Metric, B.Cu at (191.4, 65.0)
- added FB28: 470Ω, Inductor_SMD:L_0603_1608Metric, B.Cu at (110.6, 38.7)
- added FB29: 470Ω, Inductor_SMD:L_0603_1608Metric, B.Cu at (127.1, 66.3)
- added FB29: 470Ω, Inductor_SMD:L_0603_1608Metric, B.Cu at (100.1, 37.4)
- added FB29: 470Ω, Inductor_SMD:L_0603_1608Metric, B.Cu at (180.9, 63.8)
- added FB29: 470Ω, Inductor_SMD:L_0603_1608Metric, B.Cu at (154.6, 36.2)
- added FB29: 470Ω, Inductor_SMD:L_0603_1608Metric, B.Cu at (127.9, 36.7)
- added FB29: 470Ω, Inductor_SMD:L_0603_1608Metric, B.Cu at (100.1, 66.8)
- added FB29: 470Ω, Inductor_SMD:L_0603_1608Metric, B.Cu at (154.9, 64.8)
- added FB7: 470Ω, Inductor_SMD:L_0603_1608Metric, B.Cu at (99.2, 55.2)
- added FB7: 470Ω, Inductor_SMD:L_0603_1608Metric, B.Cu at (153.9, 53.2)
- added FB7: 470Ω, Inductor_SMD:L_0603_1608Metric, B.Cu at (179.9, 52.2)
- added FB7: 470Ω, Inductor_SMD:L_0603_1608Metric, B.Cu at (126.2, 54.8)
- added FB7: 470Ω, Inductor_SMD:L_0603_1608Metric, B.Cu at (153.7, 24.7)
- added FB7: 470Ω, Inductor_SMD:L_0603_1608Metric, B.Cu at (99.2, 25.9)
- added FB7: 470Ω, Inductor_SMD:L_0603_1608Metric, B.Cu at (126.9, 25.2)
- added FB9: 470Ω, Inductor_SMD:L_0603_1608Metric, B.Cu at (189.8, 61.1)
- added FB9: 470Ω, Inductor_SMD:L_0603_1608Metric, B.Cu at (136.8, 34.0)
- added FB9: 470Ω, Inductor_SMD:L_0603_1608Metric, B.Cu at (109.1, 64.1)
- added FB9: 470Ω, Inductor_SMD:L_0603_1608Metric, B.Cu at (109.1, 34.7)
- added FB9: 470Ω, Inductor_SMD:L_0603_1608Metric, B.Cu at (163.6, 33.5)
- added FB9: 470Ω, Inductor_SMD:L_0603_1608Metric, B.Cu at (136.1, 63.6)
- added FB9: 470Ω, Inductor_SMD:L_0603_1608Metric, B.Cu at (163.8, 62.1)
- added IC1: 830S21AMI-01LF, custom_components:SOIC127P600X175-8N, F.Cu at (111.5, 34.2)
- added IC1: 830S21AMI-01LF, custom_components:SOIC127P600X175-8N, F.Cu at (170.3, 35.4)
- added IC1: 830S21AMI-01LF, custom_components:SOIC127P600X175-8N, F.Cu at (184.8, 35.7)
- added IC1: 830S21AMI-01LF, custom_components:SOIC127P600X175-8N, F.Cu at (127.9, 65.7)
- added IC1: 830S21AMI-01LF, custom_components:SOIC127P600X175-8N, F.Cu at (126.8, 34.7)
- added IC1: 830S21AMI-01LF, custom_components:SOIC127P600X175-8N, F.Cu at (186.2, 67.4)
- added IC1: 830S21AMI-01LF, custom_components:SOIC127P600X175-8N, F.Cu at (157.2, 67.2)
- added IC1: 830S21AMI-01LF, custom_components:SOIC127P600X175-8N, F.Cu at (95.2, 67.2)
- added IC1: 830S21AMI-01LF, custom_components:SOIC127P600X175-8N, F.Cu at (198.8, 35.4)
- added IC1: 830S21AMI-01LF, custom_components:SOIC127P600X175-8N, F.Cu at (200.4, 67.5)
- added IC1: 830S21AMI-01LF, custom_components:SOIC127P600X175-8N, F.Cu at (155.8, 35.7)
- added IC1: 830S21AMI-01LF, custom_components:SOIC127P600X175-8N, F.Cu at (171.4, 67.4)
- added IC1: 830S21AMI-01LF, custom_components:SOIC127P600X175-8N, F.Cu at (112.2, 66.9)
- added IC1: 830S21AMI-01LF, custom_components:SOIC127P600X175-8N, F.Cu at (141.5, 34.7)
- added IC1: 830S21AMI-01LF, custom_components:SOIC127P600X175-8N, F.Cu at (142.9, 66.7)
- added IC2: 830S21AMI-01LF, custom_components:SOIC127P600X175-8N, B.Cu at (182.7, 70.4)
- added IC2: 830S21AMI-01LF, custom_components:SOIC127P600X175-8N, B.Cu at (101.9, 44.0)
- added IC2: 830S21AMI-01LF, custom_components:SOIC127P600X175-8N, B.Cu at (156.4, 42.8)
- added IC2: 830S21AMI-01LF, custom_components:SOIC127P600X175-8N, B.Cu at (129.7, 43.3)
- added IC2: 830S21AMI-01LF, custom_components:SOIC127P600X175-8N, B.Cu at (156.7, 71.4)
- added IC2: 830S21AMI-01LF, custom_components:SOIC127P600X175-8N, B.Cu at (101.9, 73.4)
- added IC2: 830S21AMI-01LF, custom_components:SOIC127P600X175-8N, B.Cu at (128.9, 72.9)
- added R10: 100, Resistor_SMD:R_0603_1608Metric, B.Cu at (102.2, 25.9)
- added R10: 100, Resistor_SMD:R_0603_1608Metric, B.Cu at (156.7, 24.7)
- added R10: 100, Resistor_SMD:R_0603_1608Metric, B.Cu at (129.2, 54.8)
- added R10: 100, Resistor_SMD:R_0603_1608Metric, B.Cu at (156.9, 53.2)
- added R10: 100, Resistor_SMD:R_0603_1608Metric, B.Cu at (102.2, 55.2)
- added R10: 100, Resistor_SMD:R_0603_1608Metric, B.Cu at (129.9, 25.2)
- added R10: 100, Resistor_SMD:R_0603_1608Metric, B.Cu at (182.9, 52.2)
- added R12: 127, Resistor_SMD:R_0603_1608Metric, B.Cu at (162.5, 44.3)
- added R12: 127, Resistor_SMD:R_0603_1608Metric, B.Cu at (188.7, 71.9)
- added R12: 127, Resistor_SMD:R_0603_1608Metric, B.Cu at (108.0, 45.6)
- added R12: 127, Resistor_SMD:R_0603_1608Metric, B.Cu at (135.7, 44.8)
- added R12: 127, Resistor_SMD:R_0603_1608Metric, B.Cu at (135.0, 74.4)
- added R12: 127, Resistor_SMD:R_0603_1608Metric, B.Cu at (108.0, 74.9)
- added R12: 127, Resistor_SMD:R_0603_1608Metric, B.Cu at (162.7, 72.9)
- added R13: 82, Resistor_SMD:R_0603_1608Metric, B.Cu at (161.2, 72.9)
- added R13: 82, Resistor_SMD:R_0603_1608Metric, B.Cu at (161.0, 44.3)
- added R13: 82, Resistor_SMD:R_0603_1608Metric, B.Cu at (106.5, 74.9)
- added R13: 82, Resistor_SMD:R_0603_1608Metric, B.Cu at (133.5, 74.4)
- added R13: 82, Resistor_SMD:R_0603_1608Metric, B.Cu at (187.2, 71.9)
- added R13: 82, Resistor_SMD:R_0603_1608Metric, B.Cu at (134.2, 44.8)
- added R13: 82, Resistor_SMD:R_0603_1608Metric, B.Cu at (106.5, 45.6)
- added R14: 100, Resistor_SMD:R_0603_1608Metric, B.Cu at (108.0, 20.9)
- added R14: 100, Resistor_SMD:R_0603_1608Metric, B.Cu at (162.7, 48.3)
- added R14: 100, Resistor_SMD:R_0603_1608Metric, B.Cu at (162.5, 19.7)
- added R14: 100, Resistor_SMD:R_0603_1608Metric, B.Cu at (135.7, 20.2)
- added R14: 100, Resistor_SMD:R_0603_1608Metric, B.Cu at (108.0, 50.3)
- added R14: 100, Resistor_SMD:R_0603_1608Metric, B.Cu at (188.7, 47.3)
- added R14: 100, Resistor_SMD:R_0603_1608Metric, B.Cu at (135.0, 49.8)
- added R15: 100, Resistor_SMD:R_0603_1608Metric, B.Cu at (190.5, 48.7)
- added R15: 100, Resistor_SMD:R_0603_1608Metric, B.Cu at (164.5, 49.7)
- added R15: 100, Resistor_SMD:R_0603_1608Metric, B.Cu at (109.8, 22.3)
- added R15: 100, Resistor_SMD:R_0603_1608Metric, B.Cu at (164.3, 21.1)
- added R15: 100, Resistor_SMD:R_0603_1608Metric, B.Cu at (109.8, 51.7)
- added R15: 100, Resistor_SMD:R_0603_1608Metric, B.Cu at (137.5, 21.6)
- added R15: 100, Resistor_SMD:R_0603_1608Metric, B.Cu at (136.8, 51.2)
- added R16: 10k, Resistor_SMD:R_0603_1608Metric, B.Cu at (103.2, 60.4)
- added R16: 10k, Resistor_SMD:R_0603_1608Metric, B.Cu at (131.0, 30.3)
- added R16: 10k, Resistor_SMD:R_0603_1608Metric, B.Cu at (103.2, 31.0)
- added R16: 10k, Resistor_SMD:R_0603_1608Metric, B.Cu at (184.0, 57.4)
- added R16: 10k, Resistor_SMD:R_0603_1608Metric, B.Cu at (158.0, 58.4)
- added R16: 10k, Resistor_SMD:R_0603_1608Metric, B.Cu at (157.7, 29.8)
- added R16: 10k, Resistor_SMD:R_0603_1608Metric, B.Cu at (130.2, 59.9)
- added R21: 127, Resistor_SMD:R_0603_1608Metric, B.Cu at (162.7, 69.9)
- added R21: 127, Resistor_SMD:R_0603_1608Metric, B.Cu at (188.7, 68.9)
- added R21: 127, Resistor_SMD:R_0603_1608Metric, B.Cu at (108.0, 42.6)
- added R21: 127, Resistor_SMD:R_0603_1608Metric, B.Cu at (162.5, 41.3)
- added R21: 127, Resistor_SMD:R_0603_1608Metric, B.Cu at (135.7, 41.8)
- added R21: 127, Resistor_SMD:R_0603_1608Metric, B.Cu at (135.0, 71.4)
- added R21: 127, Resistor_SMD:R_0603_1608Metric, B.Cu at (108.0, 71.9)
- added R22: 82, Resistor_SMD:R_0603_1608Metric, B.Cu at (134.2, 41.8)
- added R22: 82, Resistor_SMD:R_0603_1608Metric, B.Cu at (161.0, 41.3)
- added R22: 82, Resistor_SMD:R_0603_1608Metric, B.Cu at (106.5, 71.9)
- added R22: 82, Resistor_SMD:R_0603_1608Metric, B.Cu at (161.2, 69.9)
- added R22: 82, Resistor_SMD:R_0603_1608Metric, B.Cu at (133.5, 71.4)
- added R22: 82, Resistor_SMD:R_0603_1608Metric, B.Cu at (106.5, 42.6)
- added R22: 82, Resistor_SMD:R_0603_1608Metric, B.Cu at (187.2, 68.9)
- added R6: 127, Resistor_SMD:R_0603_1608Metric, F.Cu at (128.3, 40.6)
- added R6: 127, Resistor_SMD:R_0603_1608Metric, F.Cu at (129.4, 71.7)
- added R6: 127, Resistor_SMD:R_0603_1608Metric, F.Cu at (186.3, 41.6)
- added R6: 127, Resistor_SMD:R_0603_1608Metric, F.Cu at (113.0, 40.1)
- added R6: 127, Resistor_SMD:R_0603_1608Metric, F.Cu at (113.7, 72.9)
- added R6: 127, Resistor_SMD:R_0603_1608Metric, F.Cu at (157.3, 41.6)
- added R6: 127, Resistor_SMD:R_0603_1608Metric, F.Cu at (96.7, 73.2)
- added R6: 127, Resistor_SMD:R_0603_1608Metric, F.Cu at (158.7, 73.2)
- added R6: 127, Resistor_SMD:R_0603_1608Metric, F.Cu at (200.3, 41.4)
- added R6: 127, Resistor_SMD:R_0603_1608Metric, F.Cu at (201.9, 73.4)
- added R6: 127, Resistor_SMD:R_0603_1608Metric, F.Cu at (143.0, 40.6)
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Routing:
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- removed copper zone on B.Cu, net /ADC/AGND
- removed copper zone on F.Cu, net /ADC/AGND
- removed copper zone on In1.Cu, net /ADC/AGND
- removed copper zone on In2.Cu, net /ADC/AGND
- removed copper zone on B.Cu, net /ADC/DGND
- removed copper zone on F.Cu, net /ADC/DGND
- removed copper zone on In1.Cu, net /ADC/DGND
- removed copper zone on In2.Cu, net /ADC/DGND
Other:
- board size 110 x 110 mm -> 126 x 79 mm
- board text removed: "1"
- board text removed: "10"
- board text removed: "12"
- board text removed: "13"
- board text removed: "14"
- board text removed: "15"
- board text removed: "16"
- board text removed: "2"
- board text removed: "3"
- board text removed: "4"
- board text removed: "5"
- board text removed: "6"
- board text removed: "7"
- board text removed: "8"
- board text removed: "9"
- board text removed: "Epoxy Here"
